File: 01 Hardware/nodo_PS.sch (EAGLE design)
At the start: 31 parts, among them IC1 ATMEGA3208-XU, SW1 EG1213

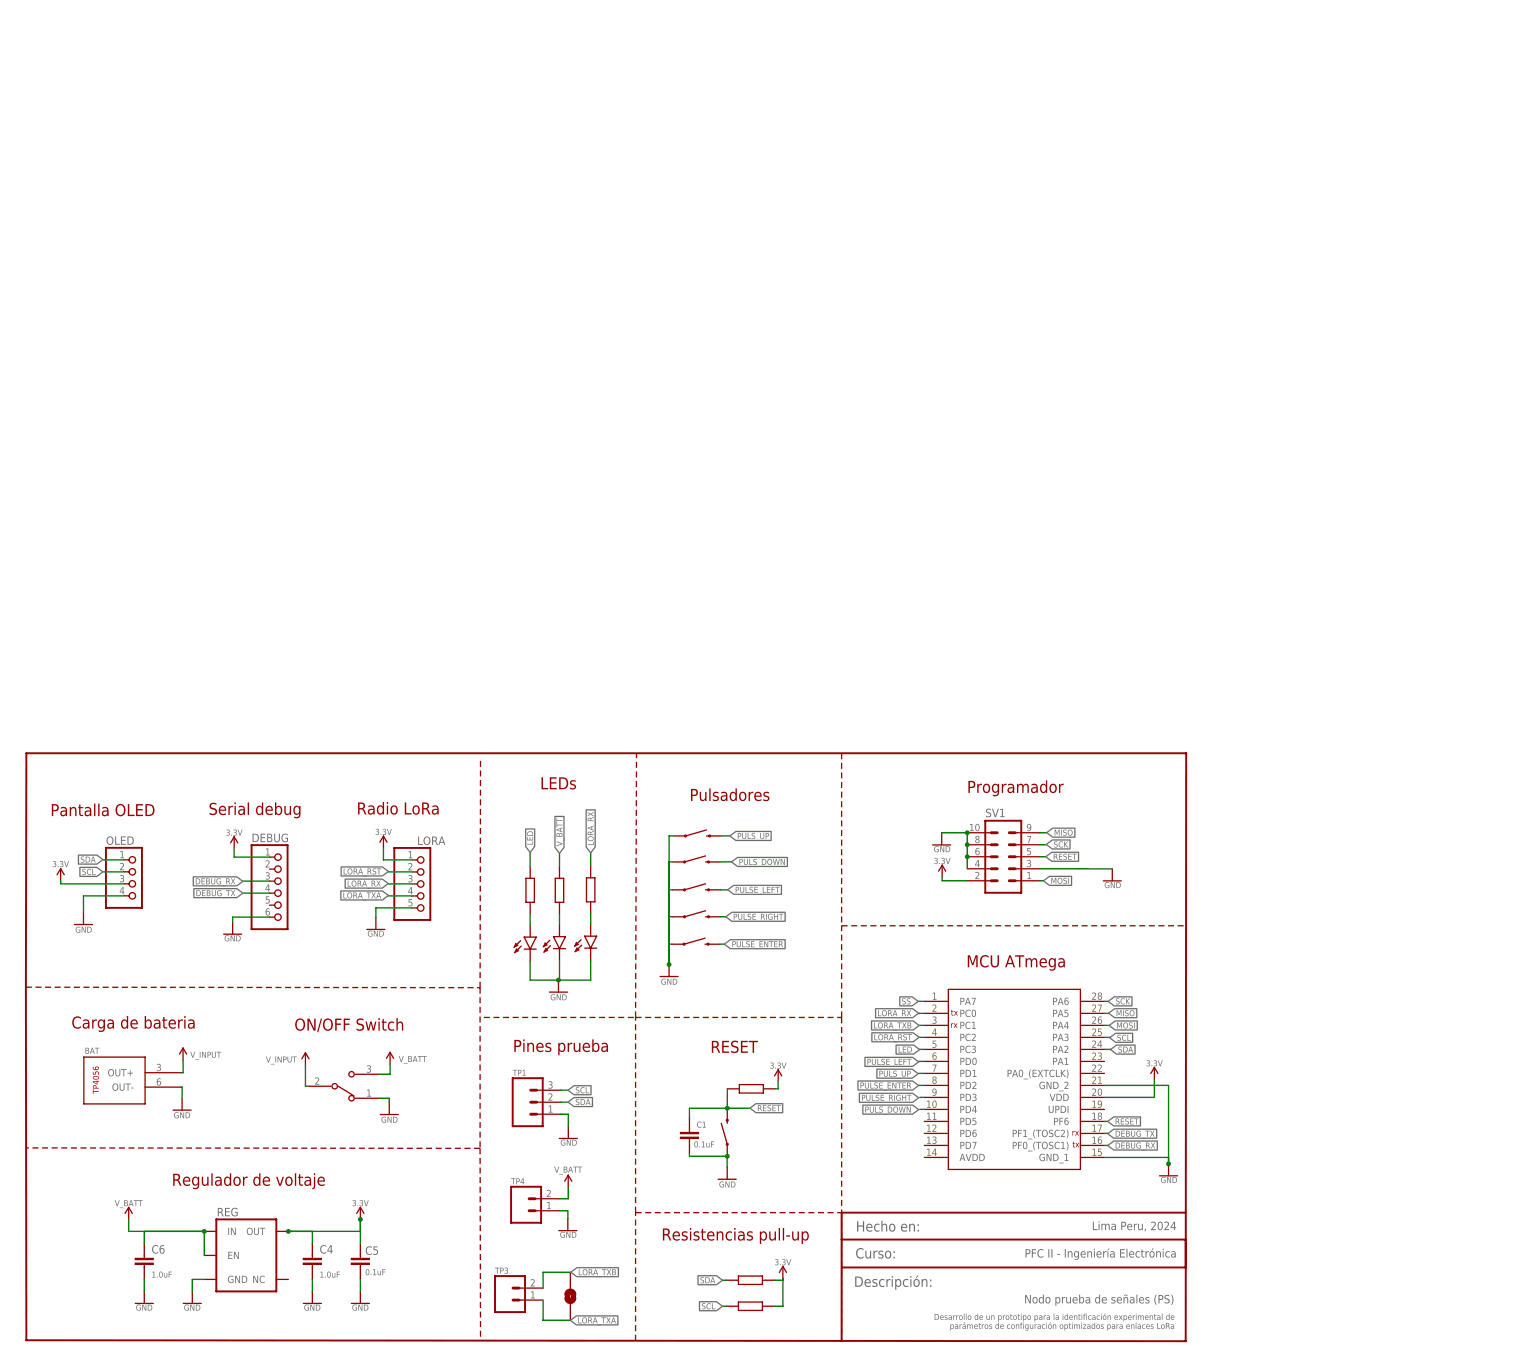
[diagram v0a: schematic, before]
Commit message: actualizacion de archivos 24-2
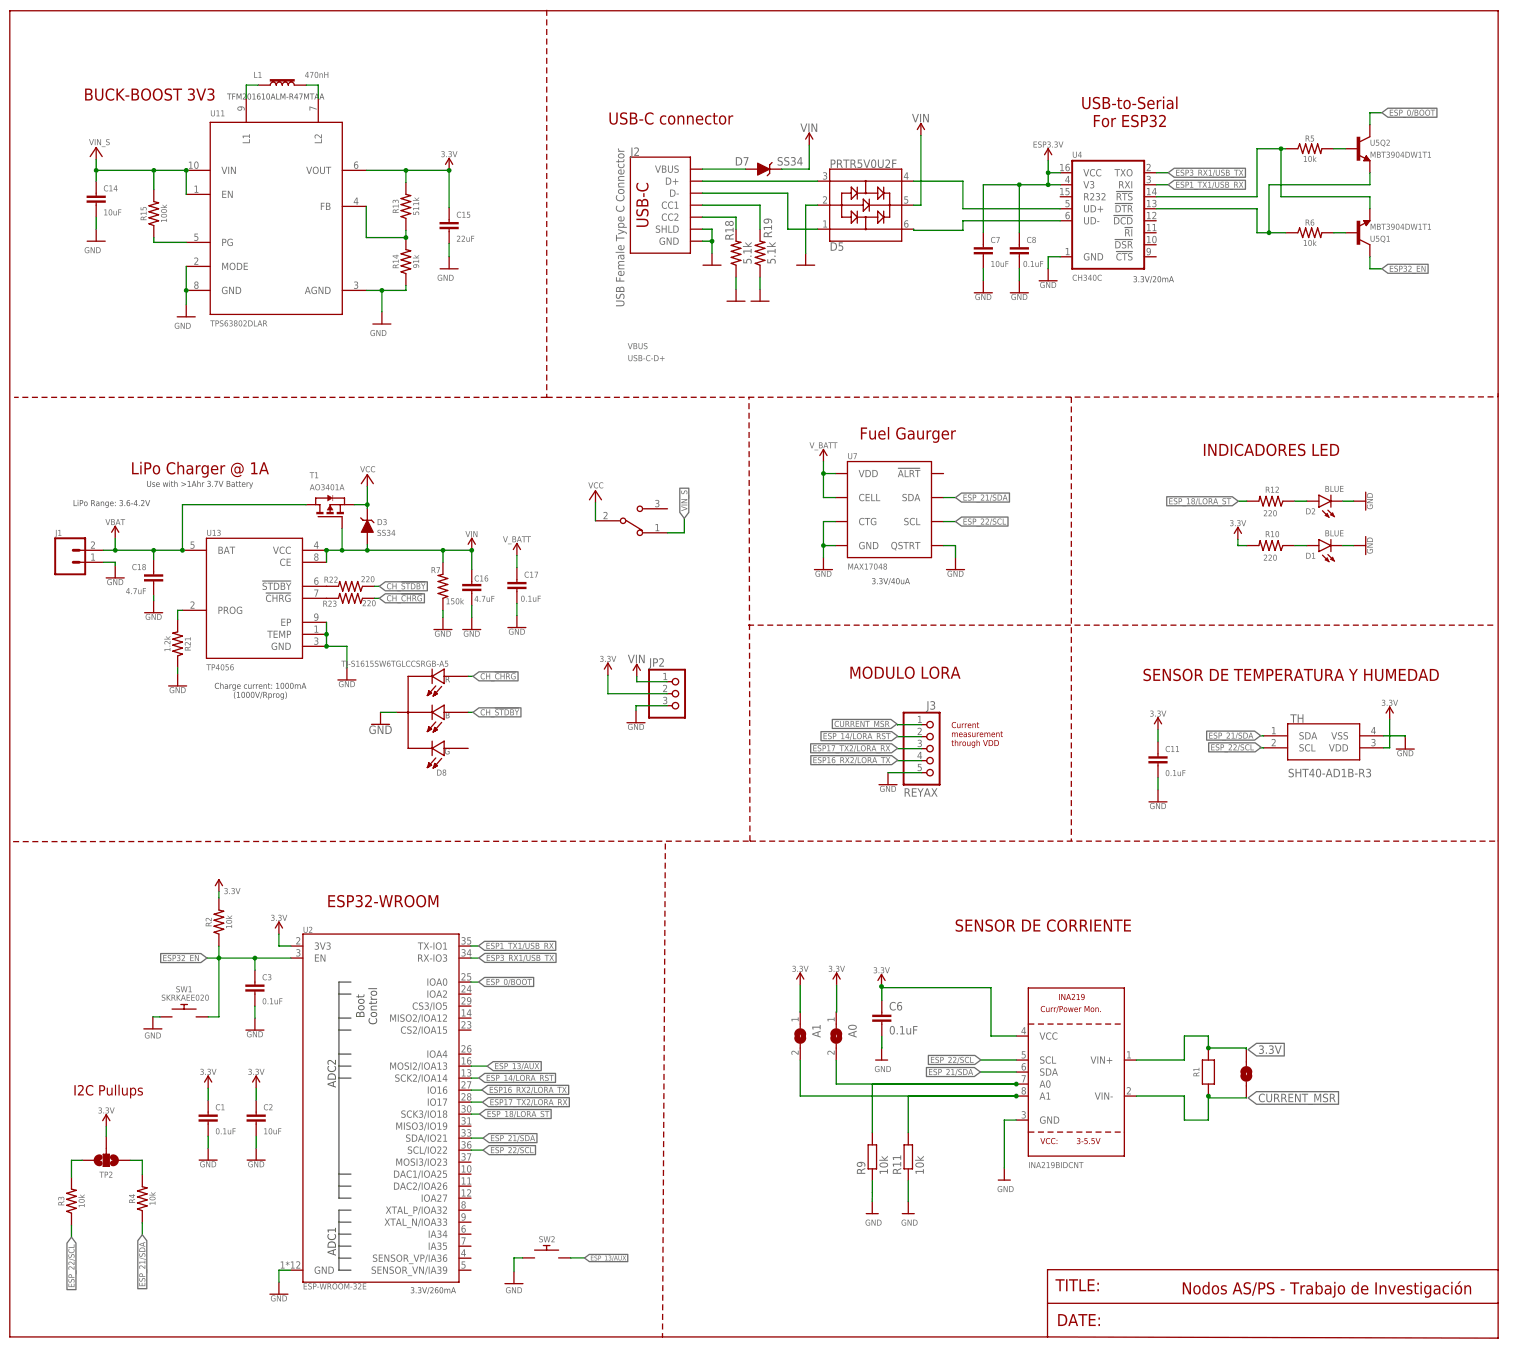
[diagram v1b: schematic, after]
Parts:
- removed BAT: TP4056MODULE, TP4056MODULE:TP4056MODULE
- removed C4: 1.0uF, SparkFun-Capacitors:1.0UF-0603-16V-10%-X7R
- removed C5: 0.1uF, SparkFun-Capacitors:0.1UF-0603-25V-5%
- removed DEBUG: (no value), pinhead:PINHD-1X6
- removed IC1: ATMEGA3208-XU, ATMEGA3208-XU:ATMEGA3208-XU
- removed LORA: REYAX, pinhead:PINHD-1X5
- removed L_ON1, L_ON2, L_ON3: LED_3MM, LED_3MM:LED_3MM
- removed OLED: (no value), pinhead:PINHD-1X4
- removed P_DOWN, P_ENTER, P_LEFT, P_RESET, P_RIGHT, P_UP: MOMENTARY-SWITCH-SPST-PTH-6.0MM, SparkFun-Switches:MOMENTARY-SWITCH-SPST-PTH-6.0MM
- removed R8: 10k, rcl:R-EU_0207/10
- removed REG: 3.3V, SparkFun-IC-Power:V_REG_AP2112K-3.3V
- removed SV1: (no value), con-harting-ml:ML10-3M
- removed TP1: (no value), SparkFun-Connectors:CONN_03
- removed TP3, TP4: (no value), SparkFun-Connectors:CONN_02
- added A0, A1: (no value), microbuilder:SOLDERJUMPERREFLOW_NOPASTE
- added C11, C17, C3, C8: 0.1uF, SparkFun-Capacitors:0.1UF-0603-25V-(+80/-20%)
- added C14: 10uF, SparkFun-Capacitors:22UF-1206-50V-10%
- added C15: 22uF, SparkFun-Capacitors:22UF-1206-50V-10%
- added C16, C18: 4.7uF, SparkFun-Capacitors:4.7UF-0603-35V-(20%)
- added C2, C7: 10uF, SparkFun-Capacitors:10UF-0603-6.3V-20%
- added D1, D2: BLUE, SparkFun-LED:LED-YELLOW0603
- added D3, D7: SS34, SparkFun-DiscreteSemi:DIODE_TVS_UNI
- added D5: PRTR5V0U2F, SparkFun-IC-Power:PRTR5V0U2F
- added D8: TJ-S1615SW6TGLCCSRGB-A5, SMD_RGB_:OSTB0603C1C
- added J1: (no value), SparkFun-Connectors:CONN_02LOCK_LONGPADS
- added J2: USB Female Type C Connector, SparkFun-Connectors:USB_C_4-LAYER_PADS
- added J3: REYAX, pinhead:PINHD-1X5
- added JP2: (no value), pinhead:PINHD-1X3
- added L1: 470nH, SparkFun-Coils:FERRITE_BEAD-0805-600Ω-100MHZ
- added R10, R12, R22, R23: 220, SparkFun-Resistors:20OHM-0603-1/10W-1%
- added R11, R9: 10k, rcl:R-EU_R0805
- added R13: 511k, SparkFun-Resistors:750KOHM-0603-1/10W-1%
- added R14: 91k, SparkFun-Resistors:750KOHM-0603-1/10W-1%
- added R15: 100k, SparkFun-Resistors:750KOHM-0603-1/10W-1%
- added R18, R19: 5.1k, SparkFun-Resistors:5.1KOHM5.1KOHM-0603-1/10W-1%
- added R21: 1.2k, SparkFun-Resistors:150KOHM-0603-1/10W-1%
- added R3, R5: 10k, SparkFun-Resistors:10KOHM-0603-1/10W-1%
- added S1: EG1213, EG1213:EG1213
- added SENSORCORRIENTE: INA219BIDCNT, microbuilder:INA219
- added SW2: SKRKAEE020, SKRKAEE020:SKRKAEE020
- added T1: AO3401A, zetex:PMOSSOT23
- added TH: SHT40-AD1B-R3, SHT40-AD1B-R3:SHT40-AD1B-R3
- added TP2: JUMPER-SMT_3_NO_NO-SILK, SparkFun-Jumpers:JUMPER-SMT_3_NO_NO-SILK
- added U11: TPS63802DLAR, TPS63802DLAR:TPS63802DLAR
- added U13: TP4056, TP4056:TP4056
- added U2: ESP-WROOM-32E, SparkFun-RF:ESP-WROOM-3232D-NARROW
- added U4: CH340C, SparkFun-IC-Comms:CH340C
- added U5: MBT3904DW1T1, SparkFun-DiscreteSemi:TRANS_NPN_DUAL-MBT3904DW1T1
- added U7: MAX17048, SparkFun-IC-Power:MAX17048DFN8
- C1: device rcl:C-EUC0603K -> SparkFun-Capacitors:0.1UF-0603-25V-(+80/-20%)
- C6: value 1.0uF -> 0.1uF; device SparkFun-Capacitors:1.0UF-0603-16V-10%-X7R -> rcl:C-EUC0805
- R1: value 68 -> 0.1/1% (PT2512FK-070R1L); device rcl:R-EU_0207/10 -> microbuilder:RESISTOR2512
- R2, R4: value 68 -> 10k; device rcl:R-EU_0207/10 -> SparkFun-Resistors:10KOHM-0603-1/10W-1%
- R6: value 1k -> 10k; device rcl:R-EU_0207/10 -> SparkFun-Resistors:10KOHM-0603-1/10W-1%
- R7: value 1k -> 150k; device rcl:R-EU_0207/10 -> SparkFun-Resistors:150KOHM-0603-1/10W-1%
- SW1: value EG1213 -> SKRKAEE020; device EG1213:EG1213 -> SKRKAEE020:SKRKAEE020
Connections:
- removed net DEBUG_RX: DEBUG.3, IC1.PF0_(TOSC1)
- removed net DEBUG_TX: DEBUG.4, IC1.PF1_(TOSC2)
- removed net LED: IC1.PC3, R2.1
- removed net LORA_RST: IC1.PC2, LORA.2
- removed net LORA_RX: IC1.PC0, LORA.3, R4.1
- removed net LORA_TXA: JP1.2, LORA.4, TP3.1
- removed net LORA_TXB: IC1.PC1, JP1.1, TP3.2
- removed net MISO: IC1.PA5, SV1.9
- removed net MOSI: IC1.PA4, SV1.1
- removed net N$2: L_ON2.A, R1.2
- removed net PULSE_ENTER: IC1.PD2, P_ENTER.2
- removed net PULSE_LEFT: IC1.PD0, P_LEFT.2
- removed net PULSE_RIGHT: IC1.PD3, P_RIGHT.2
- removed net PULS_DOWN: IC1.PD4, P_DOWN.2
- removed net PULS_UP: IC1.PD1, P_UP.2
- removed net RESET: C1.1, IC1.PF6, P_RESET.2, R8.1, SV1.5
- removed net SCK: IC1.PA6, SV1.7
- removed net SCL: IC1.PA3, OLED.2, R7.1, TP1.3
- removed net SDA: IC1.PA2, OLED.1, R6.1, TP1.2
- removed net SS: IC1.PA7
- removed net V_BATT: C6.1, R1.1, REG.EN, REG.IN, SW1.3, TP4.2
- new net ADDR0: A0.2, R9.2, SENSORCORRIENTE.A0
- new net ADDR1: A1.2, R11.2, SENSORCORRIENTE.A1
- new net CC1: J2.CC2, R18.2
- new net CC2: J2.CC1, R19.2
- new net CH_!CHRG: D8.3, R23.1
- new net CH_!STDBY: D8.2, R22.1
- new net CURRENT_MSR: J3.1, JP1.2, R1.1, SENSORCORRIENTE.VIN-
- new net ESP16_RX2/LORA_TX: J3.4, U2.IO16
- new net ESP17_TX2/LORA_RX: J3.3, U2.IO17
- new net ESP1_TX1/USB_RX: U2.TX-IO1, U4.RXI
- new net ESP32_!DTR: R6.1, U4.!DTR, U5Q2.E
- new net ESP32_!RTS: R5.1, U4.!RTS, U5Q1.E
- new net ESP32_EN: C3.1, R2.1, SW1.2, U2.EN, U5Q1.C
- new net ESP3_RX1/USB_TX: U2.RX-IO3, U4.TXO
- new net ESP_0/BOOT: U2.IOA0, U5Q2.C
- new net ESP_13/AUX: SW2.2, U2.MOSI2/IOA13
- new net ESP_14/LORA_RST: J3.2, U2.SCK2/IOA14
- new net ESP_18/LORA_ST: R12.2, U2.SCK3/IO18
- new net ESP_21/SDA: R4.1, SENSORCORRIENTE.SDA, TH.SDA, U2.SDA/IO21, U7.SDA
- new net ESP_22/SCL: R3.1, SENSORCORRIENTE.SCL, TH.SCL, U2.SCL/IO22, U7.SCL
- new net N$10: L1.2, U11.L2
- new net N$11: R22.2, U13.!STDBY
- new net N$12: R13.1, R14.2, U11.FB
- new net N$13: R23.2, U13.!CHRG
- new net N$14: R3.2, TP2.3
- new net N$15: R4.2, TP2.1
- new net N$18: R15.1, U11.PG
- new net N$24: R6.2, U5Q1.B
- new net N$25: R5.2, U5Q2.B
- new net N$31: R21.2, U13.PROG
- new net N$4: D5.6, U4.UD-
- new net N$5: D1.A, R10.1
- new net N$7: D2.A, R12.1
- new net N$8: L1.1, U11.L1
- new net USB-C-D+: D5.3, J2.D+
- new net VBAT: C17.1, C18.1, J1.2, T1.D, U13.BAT, U7.CELL, U7.VDD
- new net VBUS: D7.A, J2.VBUS
- new net VCC: D3.C, S1.2, T1.S
- new net VIN_S: C14.1, R15.2, S1.1, U11.EN, U11.VIN
- net 3.3V: now also A0.1, A1.1, C1.1, C11.1, C15.1, C2.1, C6.1, C7.1, C8.1, JP1.1, JP2.2, R1.2, R10.2, R13.2, R2.2, SENSORCORRIENTE.VCC, SENSORCORRIENTE.VIN+, TH.VDD, TP2.2, U11.VOUT, U2.3V3, U4.V3, U4.VCC; no longer C4.1, C5.2, DEBUG.1, IC1.VDD, LORA.1, OLED.3, R6.2, R7.2, R8.2, REG.OUT, SV1.2
- net GND: now also C11.2, C14.2, C15.2, C16.2, C17.2, C18.2, C2.2, C3.2, C7.2, C8.2, D1.C, D2.C, D5.2, D8.4, J1.1, J2.GND, J2.SHLD, J3.5, JP2.3, R11.1, R14.1, R18.1, R19.1, R21.1, R7.1, R9.1, SENSORCORRIENTE.GND, SW2.1, TH.VSS, U11.AGND, U11.GND, U11.MODE, U13.EP, U13.GND, U13.TEMP, U2.GND, U4.GND, U7.CTG, U7.GND, U7.QSTRT; no longer BAT.OUT-, C4.2, C5.1, DEBUG.6, IC1.GND_1, IC1.GND_2, LORA.5, L_ON1.C, L_ON2.C, L_ON3.C, OLED.4, P_DOWN.1, P_ENTER.1, P_LEFT.1, P_RESET.1, P_RIGHT.1, P_UP.1, REG.GND, SV1.10, SV1.3, SV1.4, SV1.6, SV1.8, TP1.1, TP4.1
- net N$1: now also D5.1, J2.D-; no longer L_ON3.A, R2.2
- net N$3: now also D5.4, U4.UD+; no longer L_ON1.A, R4.2
- net VIN: now also C16.1, D3.A, D5.5, D7.C, JP2.1, R7.2, T1.G, U13.CE, U13.VCC; no longer BAT.OUT+, SW1.2
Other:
- note added: "3.3V/20mA"
- note added: "3.3V/260mA"
- note added: "3.3V/40uA"
- note added: "BUCK-BOOST 3V3"
- note added: "Charge current: 1000mA (1000V/Rprog)"
- note added: "Current measurement through VDD"
- note added: "DATE:"
- note added: "ESP32-WROOM"
- note added: "Fuel Gaurger"
- note added: "I2C Pullups"
- note added: "INDICADORES LED"
- note added: "LiPo Charger @ 1A"
- note added: "LiPo Range: 3.6-4.2V"
- note added: "MODULO LORA"
- note added: "Nodos AS/PS - Trabajo de Investigación"
- note added: "SENSOR DE CORRIENTE"
- note added: "SENSOR DE TEMPERATURA Y HUMEDAD"
- note added: "TFM201610ALM-R47MTAA"
- note added: "TITLE:"
- note added: "USB-C connector"
- note added: "USB-to-Serial For ESP32"
- note added: "Use with >1Ahr 3.7V Battery"
- note removed: "Carga de bateria"
- note removed: "Curso:"
- note removed: "Desarrollo de un prototipo para la identificación experimental de parámetros de configuración optimizados para enlaces LoRa"
- note removed: "Descripción:"
- note removed: "Hecho en:"
- note removed: "LEDs"
- note removed: "Lima Peru, 2024"
- note removed: "MCU ATmega"
- note removed: "Nodo prueba de señales (PS)"
- note removed: "ON/OFF Switch"
- note removed: "PFC II - Ingeniería Electrónica"
- note removed: "Pantalla OLED"
- note removed: "Pines prueba"
- note removed: "Programador"
- note removed: "Pulsadores"
- note removed: "RESET"
- note removed: "Radio LoRa"
- note removed: "Regulador de voltaje"
- note removed: "Resistencias pull-up"
- note removed: "Serial debug"
- note removed: "rx"
- note removed: "tx"
- moved on the sheet: C1, C6
